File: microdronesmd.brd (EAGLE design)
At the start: 78.7 x 72.1 mm, 22 parts, among them Q1 SUP75N06-08, Q2 SUP75N06-08, Q3 SUP75N06-08, Q4 SUP75N06-08

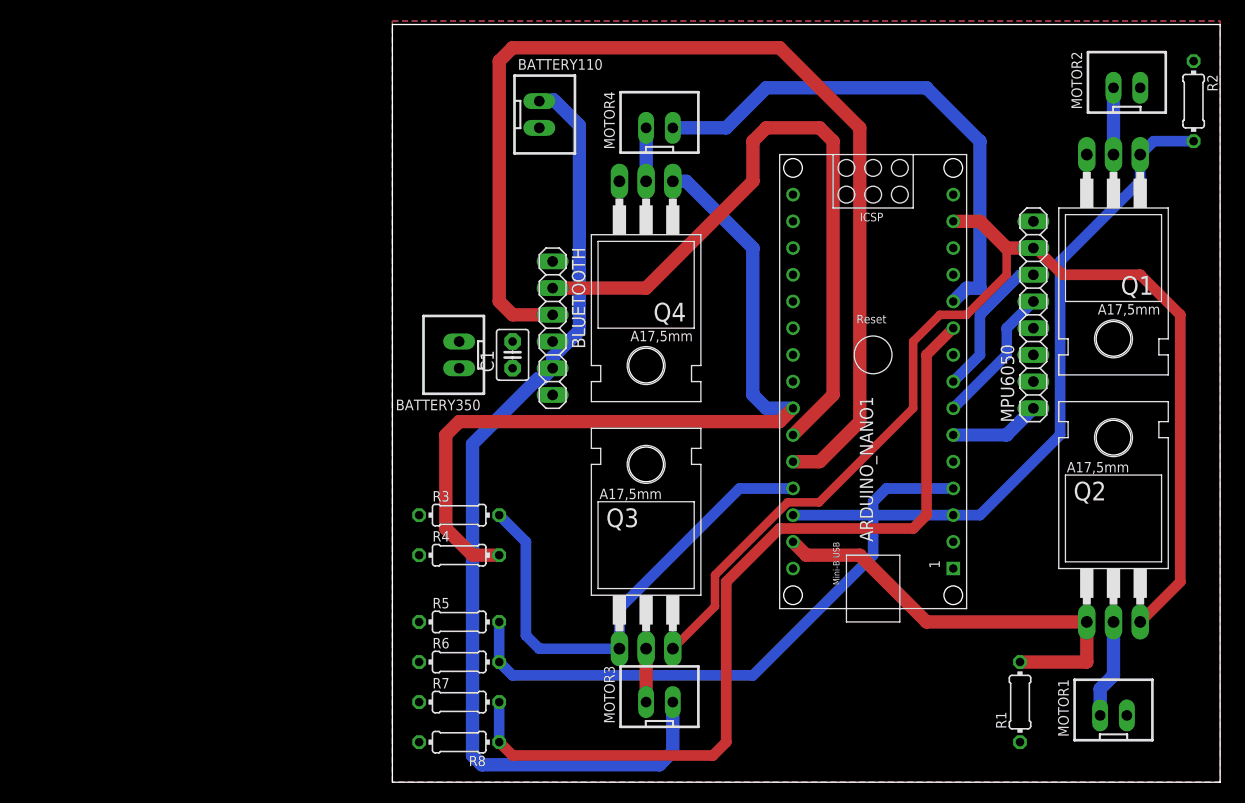
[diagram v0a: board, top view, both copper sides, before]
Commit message: Second commit
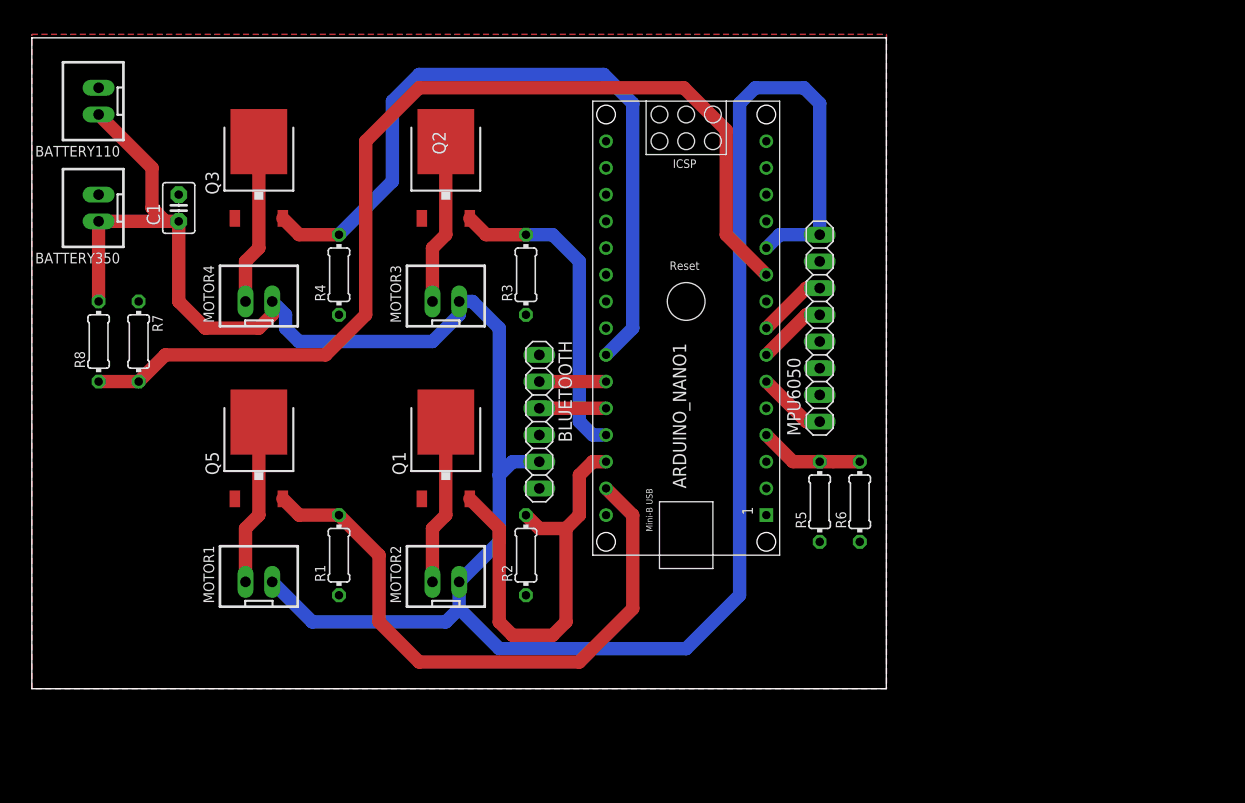
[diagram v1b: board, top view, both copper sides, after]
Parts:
- removed Q4: SUP75N06-08, transistor-fet:TO220
- added Q5: FDD4141TO252, transistor-fet:TO252
- Q1, Q2, Q3: value SUP75N06-08 -> FDD4141TO252; device transistor-fet:TO220 -> transistor-fet:TO252
- moved MOTOR1 82.3 mm to (29.2, 34.3)
- moved MOTOR2 80.0 mm to (47.0, 34.3)
- moved R2 76.8 mm to (54.6, 36.8), turned to 90 degrees
- moved Q2 73.4 mm to (47.0, 73.7)
- moved Q1 67.1 mm to (47.0, 47.0), turned to 0 degrees
- moved R1 66.3 mm to (36.8, 36.8)
- moved Q3 53.9 mm to (29.2, 73.7)
- moved R8 51.3 mm to (14.0, 57.1), turned to 90 degrees
- moved R7 45.9 mm to (17.8, 57.1), turned to 270 degrees
- moved MOTOR3 43.2 mm to (47.0, 61.0)
- moved BATTERY110 41.9 mm to (14.0, 80.0), turned to 90 degrees
- moved MOTOR4 41.5 mm to (29.2, 61.0)
- moved R6 41.0 mm to (86.4, 41.9), turned to 90 degrees
- moved BATTERY350 37.0 mm to (14.0, 69.8)
- moved R5 36.1 mm to (82.5, 41.9), turned to 90 degrees
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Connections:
- removed net GND: ARDUINO_NANO1.14, ARDUINO_NANO1.19, BATTERY110.2, BATTERY350.2, BLUETOOTH.4, C1.2, MPU6050.7, Q1.3, Q2.3, Q3.3, Q4.3, R1.1, R2.1, R3.1, R4.1, R5.1, R6.1, R7.1
- new net GND/VCC: ARDUINO_NANO1.14, ARDUINO_NANO1.19, BATTERY110.2, BATTERY350.2, BLUETOOTH.4, C1.2, MPU6050.7, Q1.1, Q2.1, Q3.1, Q5.1, R1.1, R2.1, R3.1, R4.1, R5.1, R6.1, R7.1
- net MOTOR1: now also Q5.3; no longer Q2.2
- net MOTOR2: now also Q1.3; no longer Q1.2
- net MOTOR3: now also Q2.3; no longer Q3.2
- net MOTOR4: now also Q3.3; no longer Q4.2
- net NPN1: now also Q5.2; no longer Q2.1
- net NPN2: now also Q1.2; no longer Q1.1
- net NPN3: now also Q2.2; no longer Q3.1
- net NPN4: now also Q3.2; no longer Q4.1
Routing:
- net GND: track 113.1 -> 0.00 mm
- net TXD: track 102.3 -> 6.35 mm
- net VCC: track 144.1 -> 231.2 mm
- net RXD: track 65.3 -> 6.35 mm
- net A0: track 57.9 -> 9.94 mm
- net NPN2: track 64.0 -> 42.2 mm
- net NPN1: track 41.3 -> 58.0 mm
- net NPN3: track 47.0 -> 30.4 mm
- net A6: track 82.2 -> 97.9 mm
- net MOTOR3: track 5.08 -> 15.7 mm
- net MOTOR4: track 5.08 -> 15.7 mm
- net MOTOR2: track 6.35 -> 15.7 mm
- net SCL: track 14.1 -> 6.66 mm
- net NPN4: track 77.7 -> 70.8 mm
- net SDA: track 13.3 -> 6.66 mm
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- added copper zone on layer 1, net GND/VCC
- added copper zone on layer 16, net GND/VCC
- removed copper zone on layer 16, net GND
- removed copper zone on layer 1, net VCC
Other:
- board size 78.7 x 72.1 mm -> 81.3 x 61.9 mm
